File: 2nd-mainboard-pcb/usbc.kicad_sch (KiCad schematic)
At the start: 12 parts, among them P1 USB_C_Plug_USB2.0, U5 FT232RL, U6 PTS647SM38SMTR2LFS

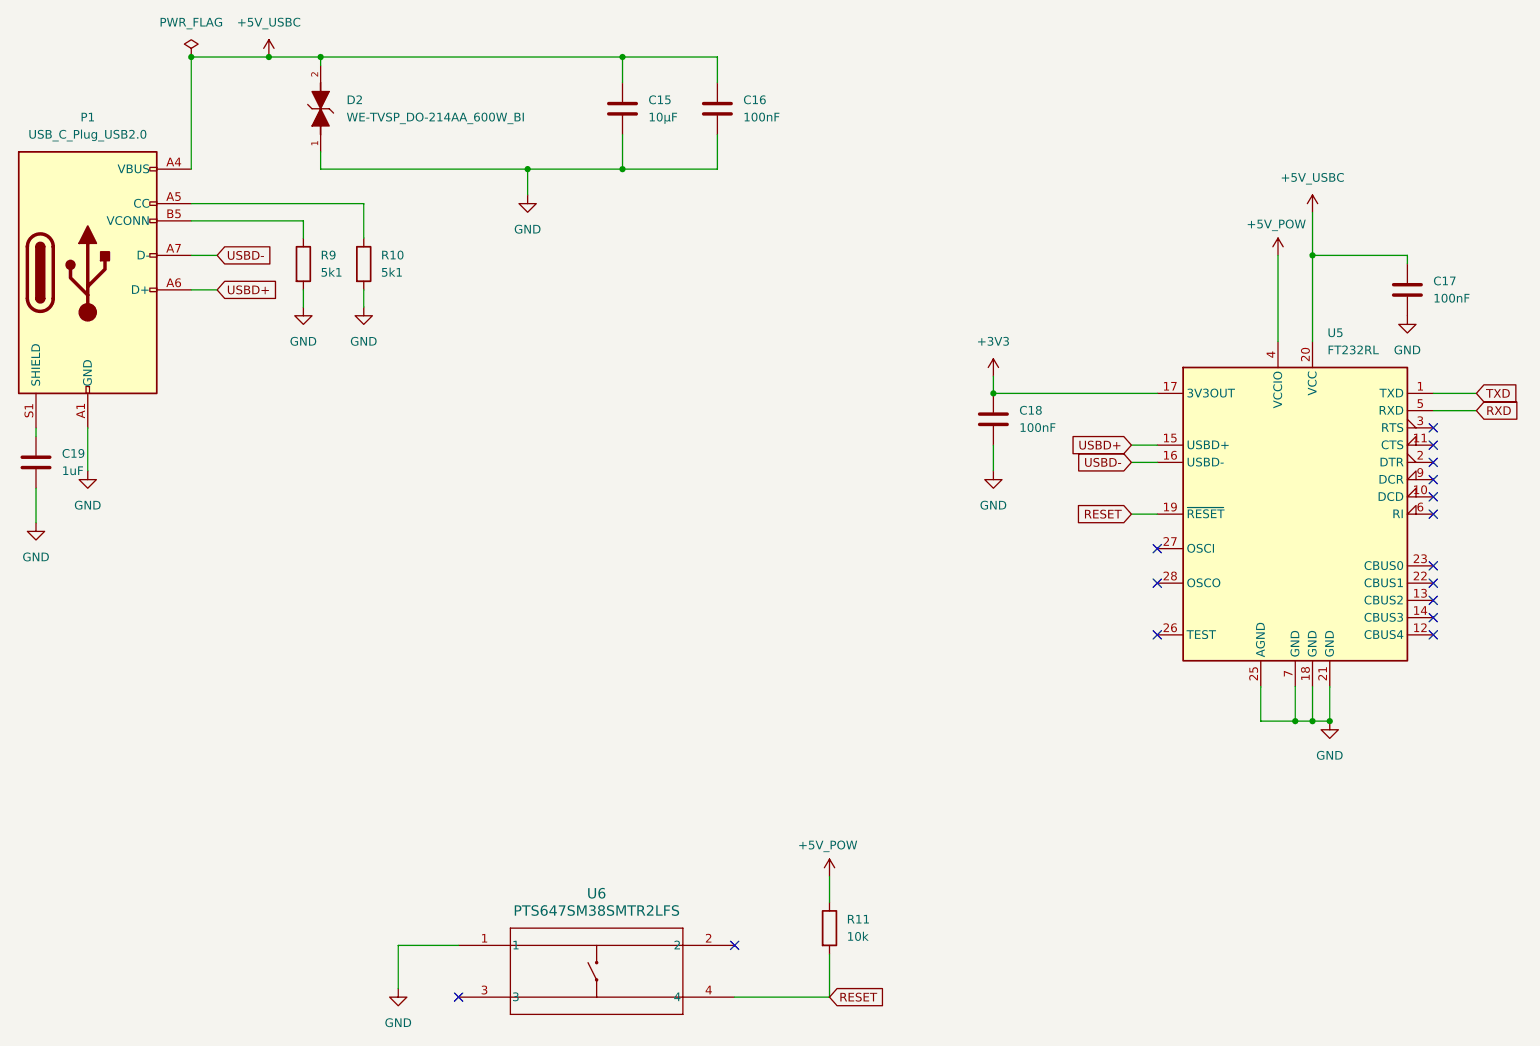
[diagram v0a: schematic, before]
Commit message: mehr positioning
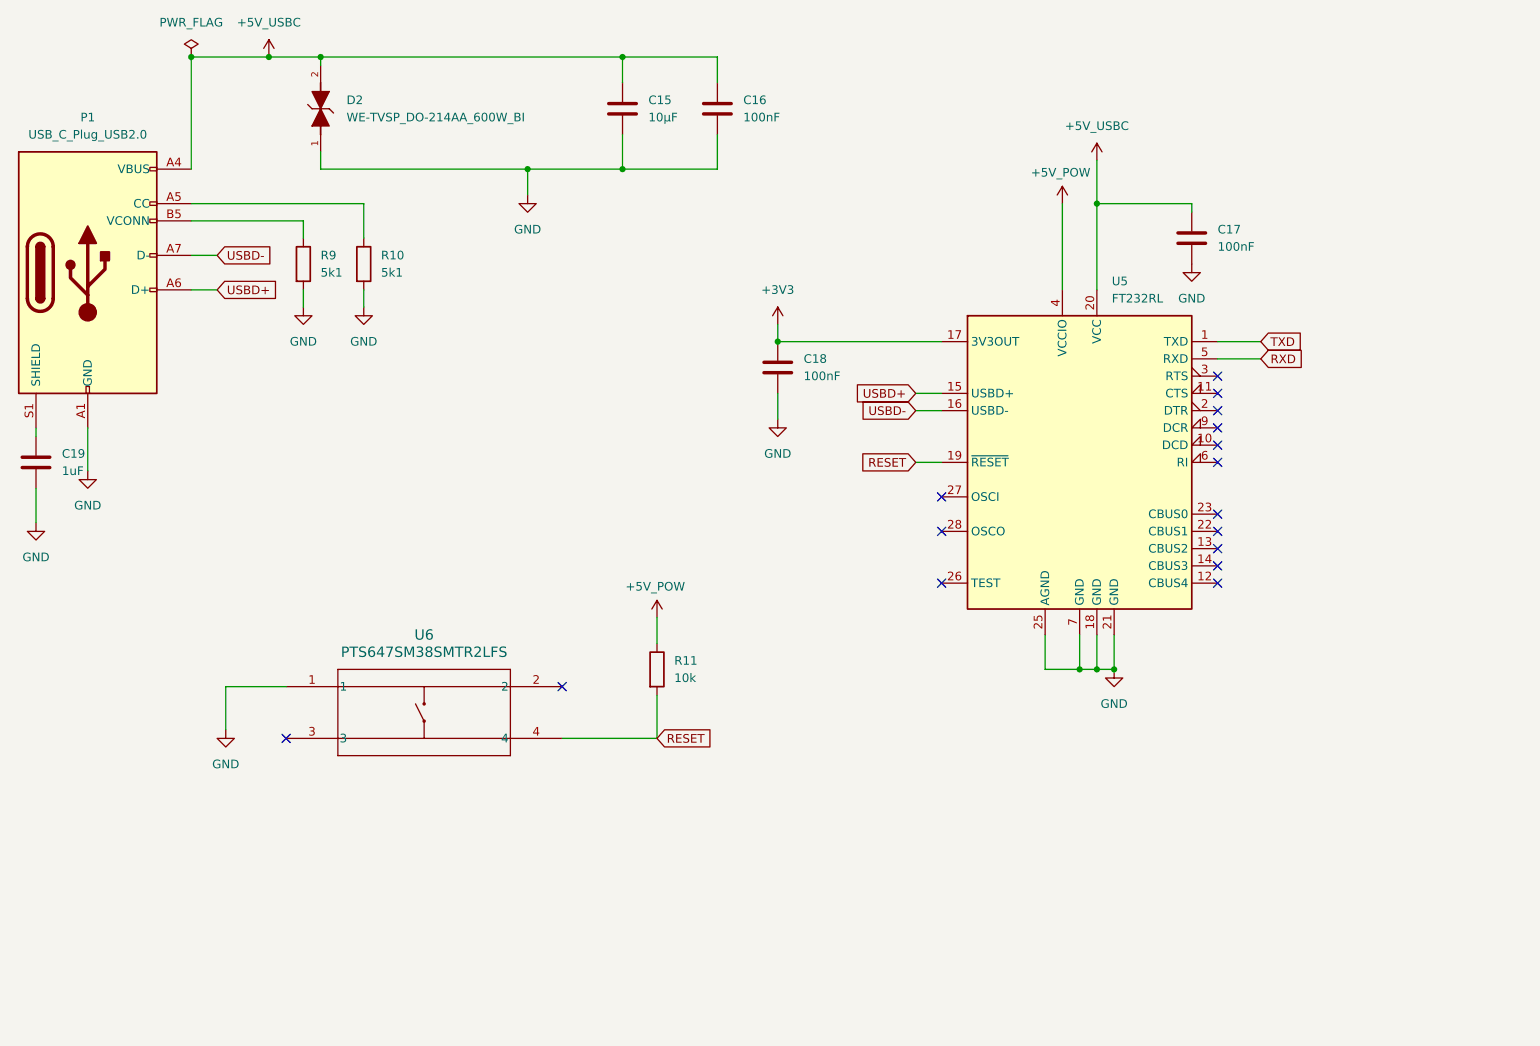
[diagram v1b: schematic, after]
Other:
- moved on the sheet: C17, C18, R11, U5, U6
